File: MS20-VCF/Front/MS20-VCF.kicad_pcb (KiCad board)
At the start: 2 copper layers, 40 x 133 mm, 4 parts

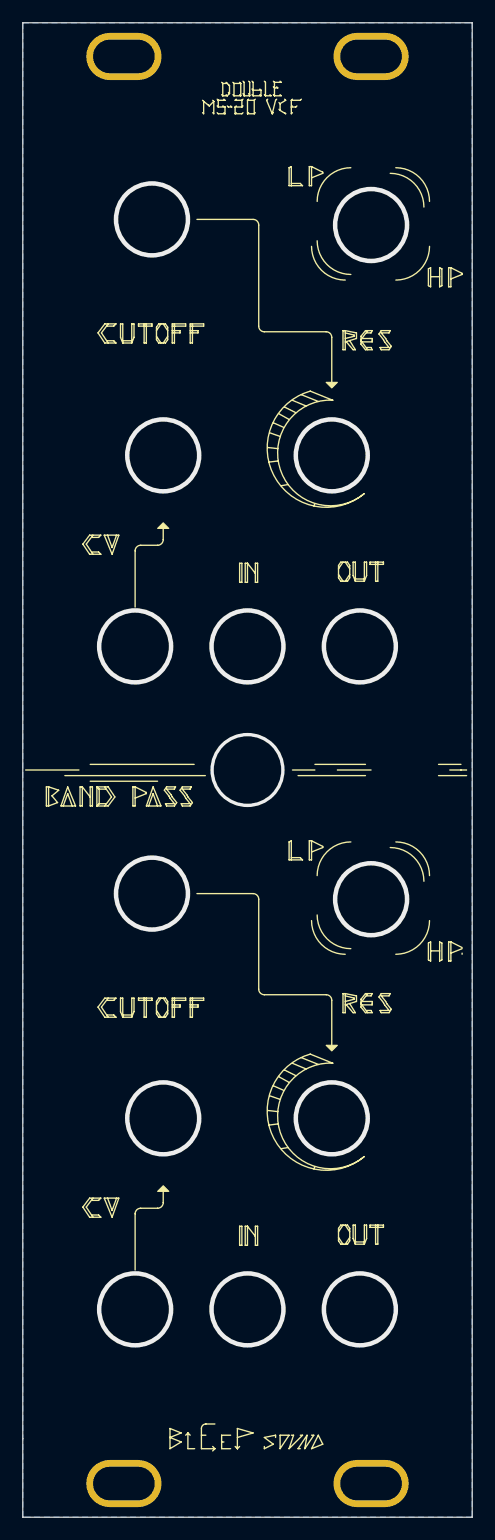
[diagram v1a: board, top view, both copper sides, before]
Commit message: Update gerber MS20-VCF
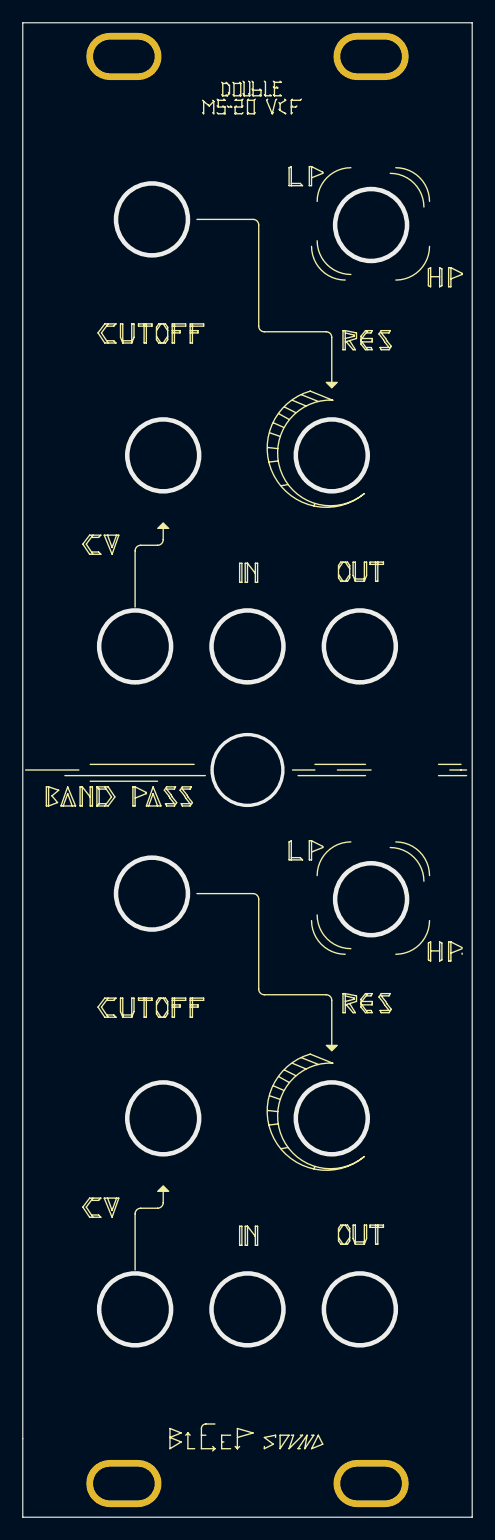
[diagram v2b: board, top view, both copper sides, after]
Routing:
- removed copper zone on B.Cu, net GND
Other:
- net class Default removed
- net class Power removed
